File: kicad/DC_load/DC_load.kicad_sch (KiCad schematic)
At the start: 4 parts

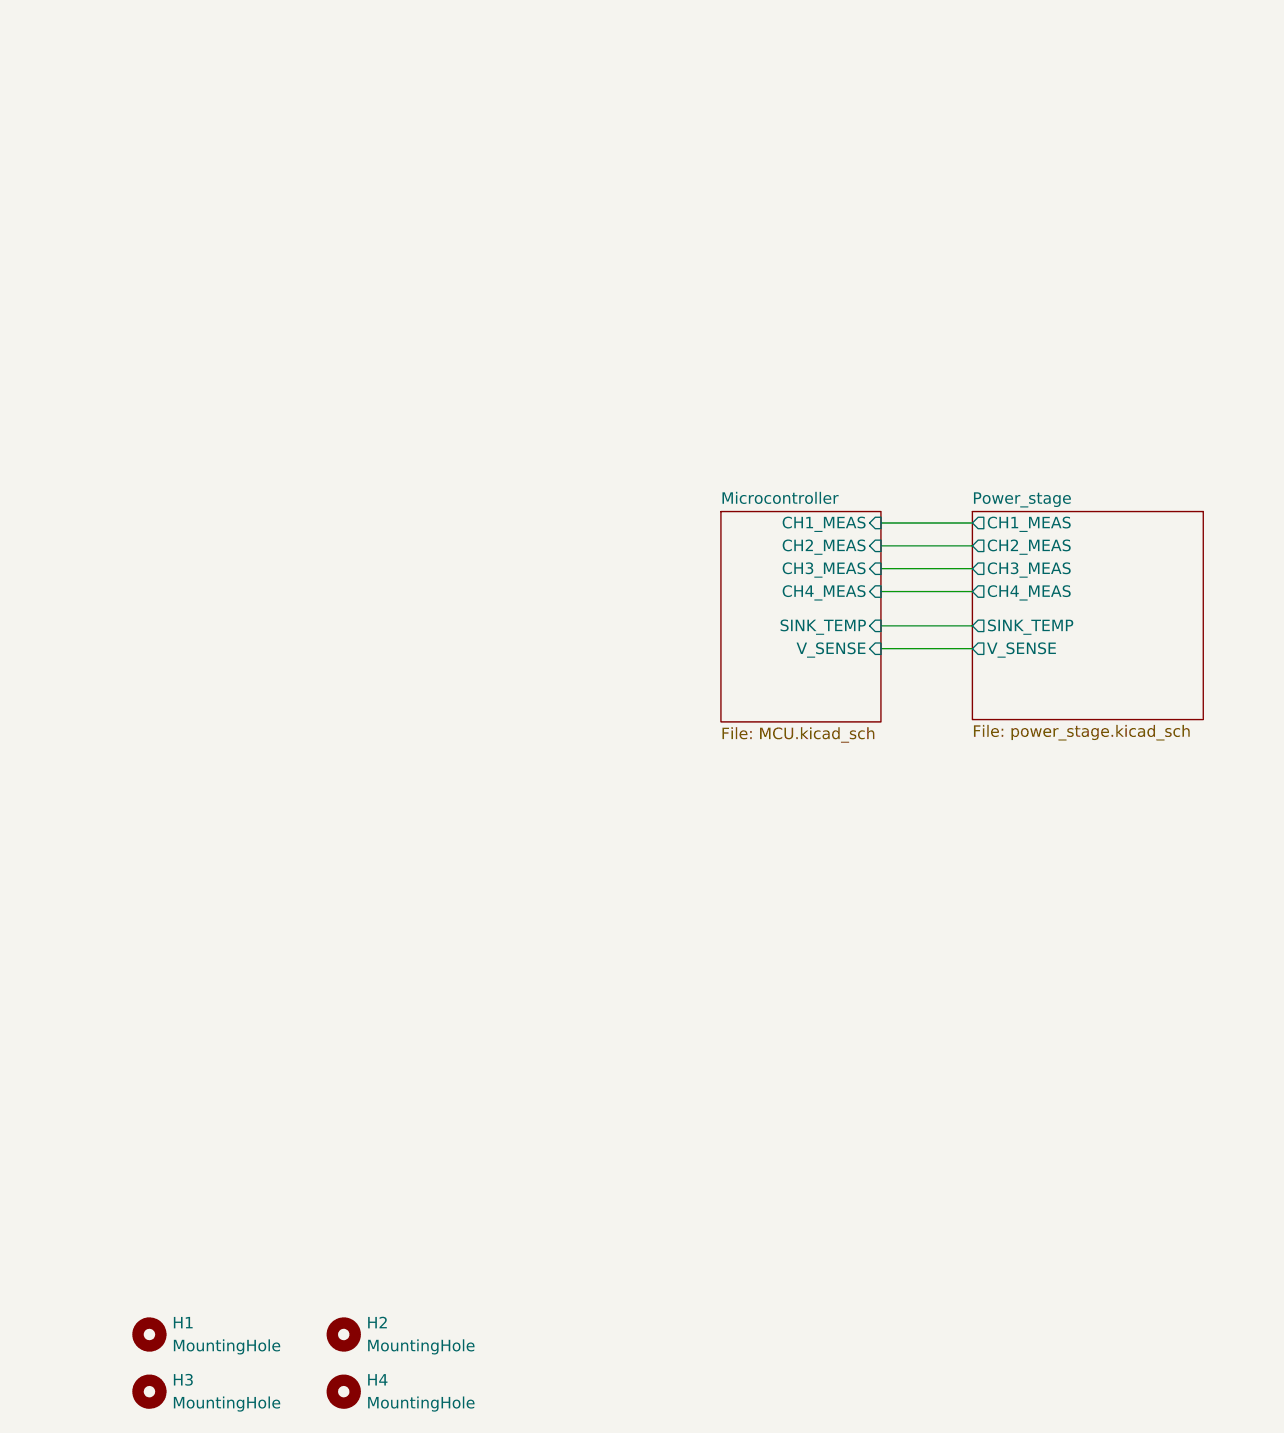
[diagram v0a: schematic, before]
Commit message: Ready for production.
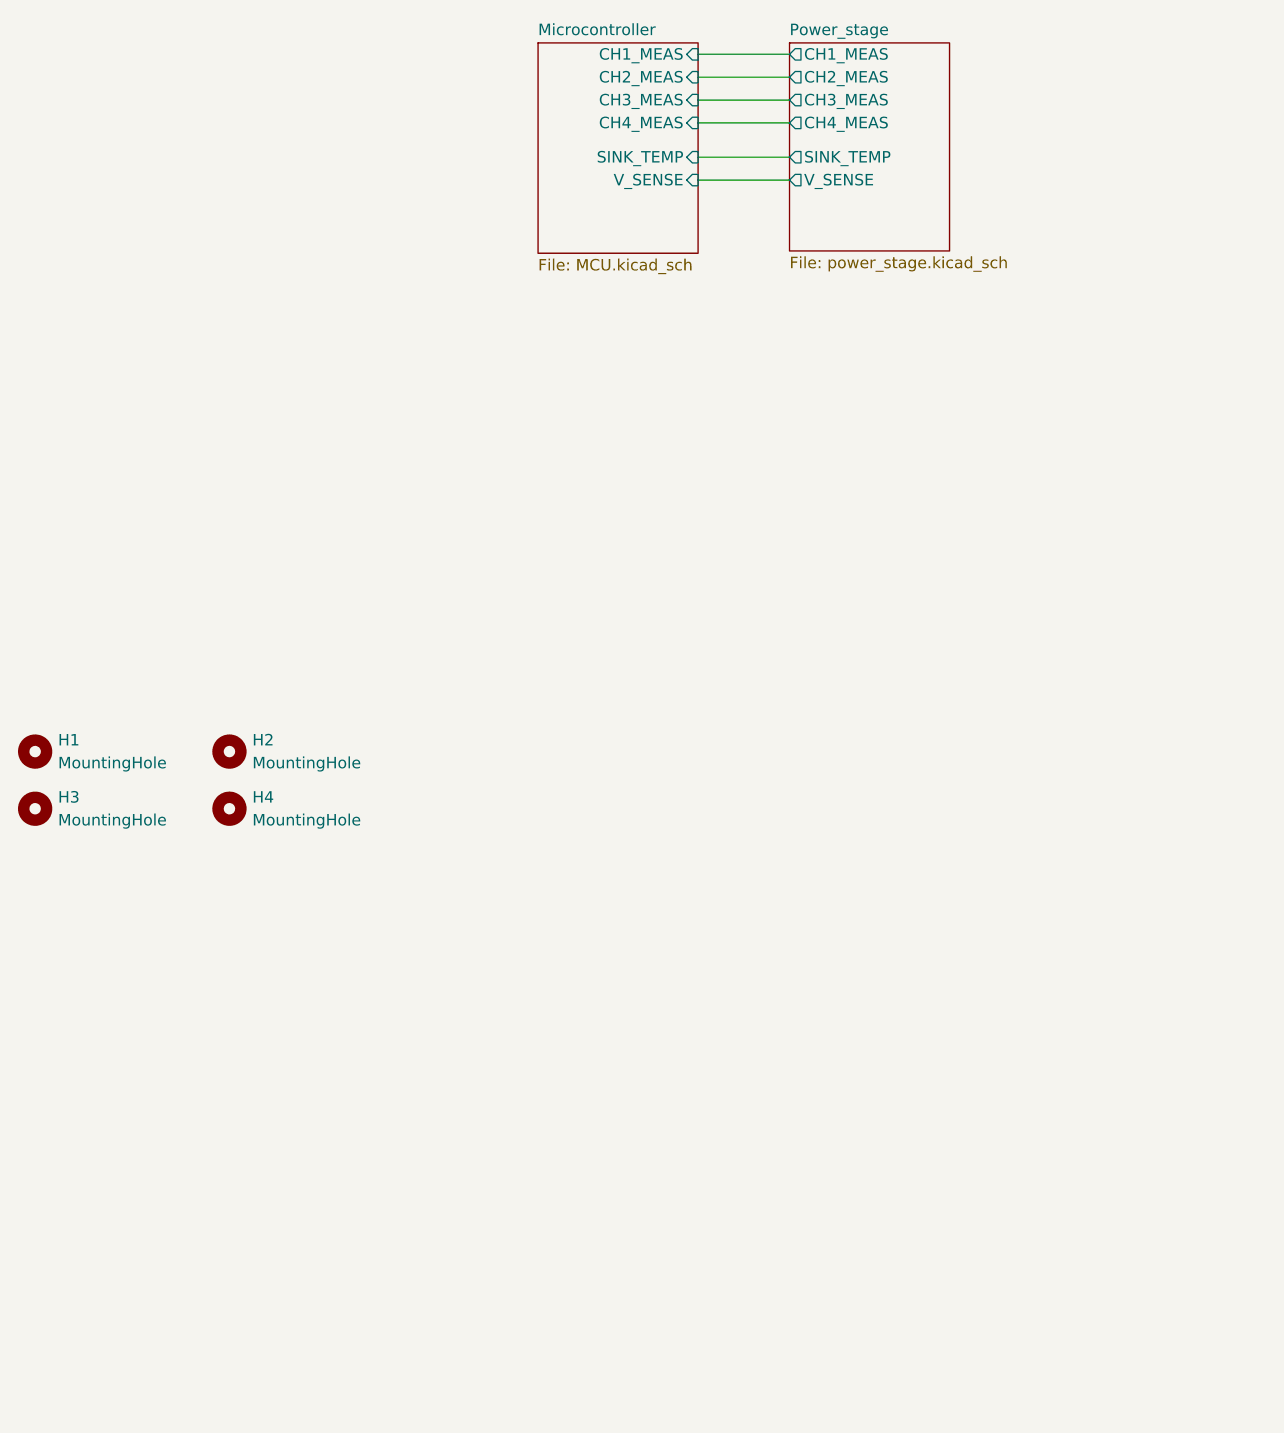
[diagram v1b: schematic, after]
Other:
- title: (none) -> DC load
- moved on the sheet: H1, H2, H3, H4
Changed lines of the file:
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@@
 	(generator "eeschema")
 	(generator_version "9.0")
-	(paper "A4")
-	(wire
-		(pts
-			(xy 124.46 110.49) (xy 134.62 110.49)
-		)
-		(stroke
-			(width 0)
-			(type default)
-		)
-	)
-	(wire
-		(pts
-			(xy 124.46 99.06) (xy 134.62 99.06)
-		)
-		(stroke
-			(width 0)
-			(type default)
-		)
-	)
-	(wire
-		(pts
-			(xy 124.46 101.6) (xy 134.62 101.6)
-		)
-		(stroke
-			(width 0)
-			(type default)
-		)
-	)
-	(wire
-		(pts
-			(xy 124.46 107.95) (xy 134.62 107.95)
-		)
-		(stroke
-			(width 0)
-			(type default)
-		)
-	)
-	(wire
-		(pts
-			(xy 124.46 104.14) (xy 134.62 104.14)
-		)
-		(stroke
-			(width 0)
-			(type default)
-		)
-	)
-	(wire
-		(pts
-			(xy 124.46 96.52) (xy 134.62 96.52)
+	(paper "A5")
+	(title_block
+		(title "DC load")
+	)
+	(wire
+		(pts
+			(xy 104.14 58.42) (xy 114.3 58.42)
+		)
+		(stroke
+			(width 0)
+			(type default)
+		)
+	)
+	(wire
+		(pts
+			(xy 104.14 46.99) (xy 114.3 46.99)
+		)
+		(stroke
+			(width 0)
+			(type default)
+		)
+	)
+	(wire
+		(pts
+			(xy 104.14 49.53) (xy 114.3 49.53)
+		)
+		(stroke
+			(width 0)
+			(type default)
+		)
+	)
+	(wire
+		(pts
+			(xy 104.14 55.88) (xy 114.3 55.88)
+		)
+		(stroke
+			(width 0)
+			(type default)
+		)
+	)
+	(wire
+		(pts
+			(xy 104.14 52.07) (xy 114.3 52.07)
+		)
+		(stroke
+			(width 0)
+			(type default)
+		)
+	)
+	(wire
+		(pts
+			(xy 104.14 44.45) (xy 114.3 44.45)
 		)
 		(stroke
@@
 	(symbol
 		(lib_id "Mechanical:MountingHole")
-		(at 43.18 186.69 0)
+		(at 30.48 121.92 0)
 		(unit 1)
 		(exclude_from_sim no)
@@
 		(fields_autoplaced yes)
 		(property "Reference" "H1"
-			(at 45.72 185.4199 0)
+			(at 33.02 120.6499 0)
 			(effects
 				(font
@@
 		)
 		(property "Value" "MountingHole"
-			(at 45.72 187.9599 0)
+			(at 33.02 123.1899 0)
 			(effects
 				(font
@@
 		)
 		(property "Footprint" "DC_load:M3_hole_with_spacer"
-			(at 43.18 186.69 0)
+			(at 30.48 121.92 0)
 			(effects
 				(font
@@
 		)
 		(property "Datasheet" "~"
-			(at 43.18 186.69 0)
+			(at 30.48 121.92 0)
 			(effects
 				(font
@@
 		)
 		(property "Description" "Mounting Hole without connection"
-			(at 43.18 186.69 0)
+			(at 30.48 121.92 0)
 			(effects
 				(font
@@
 	(symbol
 		(lib_id "Mechanical:MountingHole")
-		(at 64.77 186.69 0)
+		(at 52.07 121.92 0)
 		(unit 1)
 		(exclude_from_sim no)
@@
 		(fields_autoplaced yes)
 		(property "Reference" "H2"
-			(at 67.31 185.4199 0)
+			(at 54.61 120.6499 0)
 			(effects
 				(font
@@
 		)
 		(property "Value" "MountingHole"
-			(at 67.31 187.9599 0)
+			(at 54.61 123.1899 0)
 			(effects
 				(font
@@
 		)
 		(property "Footprint" "DC_load:M3_hole_with_spacer"
-			(at 64.77 186.69 0)
+			(at 52.07 121.92 0)
 			(effects
 				(font
@@
 		)
 		(property "Datasheet" "~"
-			(at 64.77 186.69 0)
+			(at 52.07 121.92 0)
 			(effects
 				(font
@@
 		)
 		(property "Description" "Mounting Hole without connection"
-			(at 64.77 186.69 0)
+			(at 52.07 121.92 0)
 			(effects
 				(font
@@
 	(symbol
 		(lib_id "Mechanical:MountingHole")
-		(at 43.18 193.04 0)
+		(at 30.48 128.27 0)
 		(unit 1)
 		(exclude_from_sim no)
@@
 		(fields_autoplaced yes)
 		(property "Reference" "H3"
-			(at 45.72 191.7699 0)
+			(at 33.02 126.9999 0)
 			(effects
 				(font
@@
 		)
 		(property "Value" "MountingHole"
-			(at 45.72 194.3099 0)
+			(at 33.02 129.5399 0)
 			(effects
 				(font
@@
 		)
 		(property "Footprint" "DC_load:M3_hole_with_spacer"
-			(at 43.18 193.04 0)
+			(at 30.48 128.27 0)
 			(effects
 				(font
@@
 		)
 		(property "Datasheet" "~"
-			(at 43.18 193.04 0)
+			(at 30.48 128.27 0)
 			(effects
 				(font
@@
 		)
 		(property "Description" "Mounting Hole without connection"
-			(at 43.18 193.04 0)
+			(at 30.48 128.27 0)
 			(effects
 				(font
@@
 	(symbol
 		(lib_id "Mechanical:MountingHole")
-		(at 64.77 193.04 0)
+		(at 52.07 128.27 0)
 		(unit 1)
 		(exclude_from_sim no)
@@
 		(fields_autoplaced yes)
 		(property "Reference" "H4"
-			(at 67.31 191.7699 0)
+			(at 54.61 126.9999 0)
 			(effects
 				(font
@@
 		)
 		(property "Value" "MountingHole"
-			(at 67.31 194.3099 0)
+			(at 54.61 129.5399 0)
 			(effects
 				(font
@@
 		)
 		(property "Footprint" "DC_load:M3_hole_with_spacer"
-			(at 64.77 193.04 0)
+			(at 52.07 128.27 0)
 			(effects
 				(font
@@
 		)
 		(property "Datasheet" "~"
-			(at 64.77 193.04 0)
+			(at 52.07 128.27 0)
 			(effects
 				(font
@@
 		)
 		(property "Description" "Mounting Hole without connection"
-			(at 64.77 193.04 0)
+			(at 52.07 128.27 0)
 			(effects
 				(font
@@
 	)
 	(sheet
-		(at 106.68 95.25)
+		(at 86.36 43.18)
 		(size 17.78 23.368)
 		(exclude_from_sim no)
@@
 		)
 		(property "Sheetname" "Microcontroller"
-			(at 106.68 94.5384 0)
+			(at 86.36 42.4684 0)
 			(effects
 				(font
@@
 		)
 		(property "Sheetfile" "MCU.kicad_sch"
-			(at 106.68 119.2026 0)
+			(at 86.36 67.1326 0)
 			(effects
 				(font
@@
 		)
 		(pin "CH1_MEAS" input
-			(at 124.46 96.52 0)
+			(at 104.14 44.45 0)
 			(effects
 				(font
@@
 		)
 		(pin "CH4_MEAS" input
-			(at 124.46 104.14 0)
+			(at 104.14 52.07 0)
 			(effects
 				(font
@@
 		)
 		(pin "CH2_MEAS" input
-			(at 124.46 99.06 0)
+			(at 104.14 46.99 0)
 			(effects
 				(font
@@
 		)
 		(pin "CH3_MEAS" input
-			(at 124.46 101.6 0)
+			(at 104.14 49.53 0)
 			(effects
 				(font
@@
 		)
 		(pin "SINK_TEMP" input
-			(at 124.46 107.95 0)
+			(at 104.14 55.88 0)
 			(effects
 				(font
@@
 		)
 		(pin "V_SENSE" input
-			(at 124.46 110.49 0)
+			(at 104.14 58.42 0)
 			(effects
 				(font
@@
 	)
 	(sheet
-		(at 134.62 95.25)
-		(size 25.654 23.114)
+		(at 114.3 43.18)
+		(size 17.78 23.114)
 		(exclude_from_sim no)
 		(in_bom yes)
@@
 		)
 		(property "Sheetname" "Power_stage"
-			(at 134.62 94.5384 0)
+			(at 114.3 42.4684 0)
 			(effects
 				(font
@@
 		)
 		(property "Sheetfile" "power_stage.kicad_sch"
-			(at 134.62 118.9486 0)
+			(at 114.3 66.8786 0)
 			(effects
 				(font
@@
 		)
 		(pin "CH4_MEAS" output
-			(at 134.62 104.14 180)
+			(at 114.3 52.07 180)
 			(effects
 				(font
@@
 		)
 		(pin "CH1_MEAS" output
-			(at 134.62 96.52 180)
+			(at 114.3 44.45 180)
 			(effects
 				(font
@@
 		)
 		(pin "CH3_MEAS" output
-			(at 134.62 101.6 180)
+			(at 114.3 49.53 180)
 			(effects
 				(font
@@
 		)
 		(pin "CH2_MEAS" output
-			(at 134.62 99.06 180)
+			(at 114.3 46.99 180)
 			(effects
 				(font
@@
 		)
 		(pin "SINK_TEMP" output
-			(at 134.62 107.95 180)
+			(at 114.3 55.88 180)
 			(effects
 				(font
@@
 		)
 		(pin "V_SENSE" output
-			(at 134.62 110.49 180)
-			(effects
-				(font
+			(at 114.3 58.42 180)
+			(effects
+				(font
